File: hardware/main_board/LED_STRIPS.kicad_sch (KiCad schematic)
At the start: 7 parts, among them IC801 SN74AHCT125DBR, J802 Conn_01x03_Pin

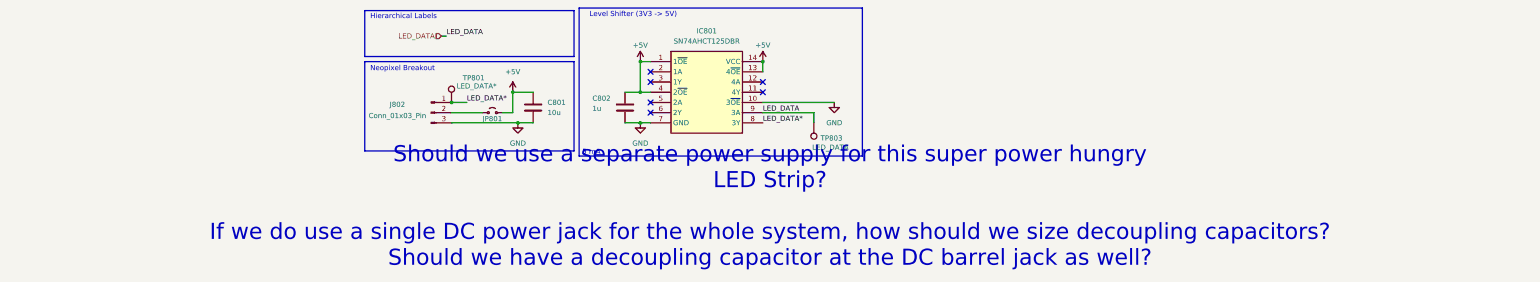
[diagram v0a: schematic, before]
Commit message: bom
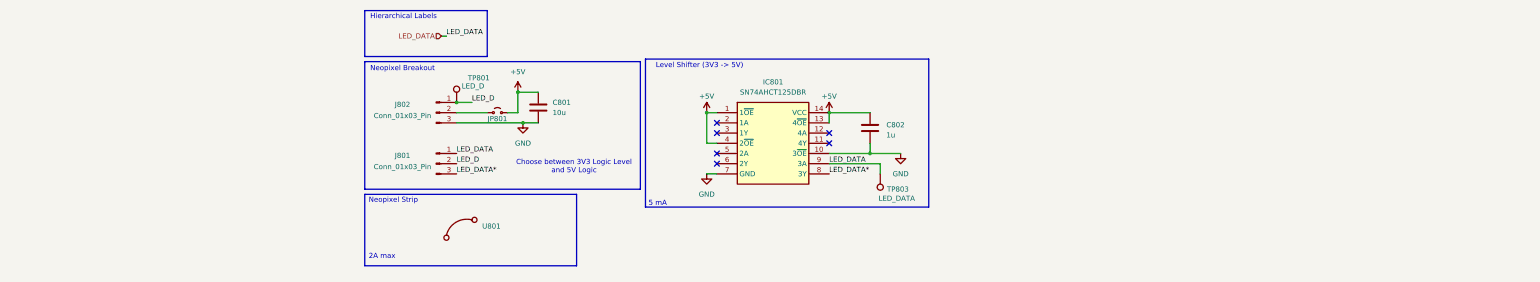
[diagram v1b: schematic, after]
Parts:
- added J801: Conn_01x03_Pin, Connector_PinHeader_2.54mm:PinHeader_1x03_P2.54mm_Vertical, symbol Connector:Conn_01x03_Pin
- added U801: ~, symbol SamacSys_Parts:led_strip
- J802, JP801: now left out of the parts list
- TP801: value LED_DATA* -> LED_D
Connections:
- net LED_DATA: now also J801.1 (Pin_1)
- net LED_DATA*: now also J801.3 (Pin_3); no longer J802.1 (Pin_1), TP801.1
- new net LED_D: J801.2 (Pin_2), J802.1 (Pin_1), TP801.1
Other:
- note added: "2A max"
- note added: "Choose between 3V3 Logic Level and 5V Logic"
- note added: "Neopixel Strip"
- note removed: "Should we use a separate power supply for this super power hungry LED Strip? If we do use a single DC power jack for the whole system, how should we size decoupling capacitors? Should we have a decoupling capacitor at the DC barrel jack as well?"
- moved on the sheet: C801, C802, IC801, J802, JP801, TP801, TP803
